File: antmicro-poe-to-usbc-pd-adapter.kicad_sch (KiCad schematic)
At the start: 93 parts, among them J1 Bus_RJ45_5-2337992-8, J2 Bus_RJ45_5-2337992-8, J3 USB-C_GCT_USB4105-GF-A, Q1 PJE138K, U1 TPS2372-3RGWR, U2 LV14540DDAR, U3 INA230AIRGTR, U4 IEA48003A280V-001-R, U5 FT4232H_VQFN, U6 TPS65987DDHRSHR, U7 LV14540DDAR, Y1 Resonator_12MHz_ABM8G

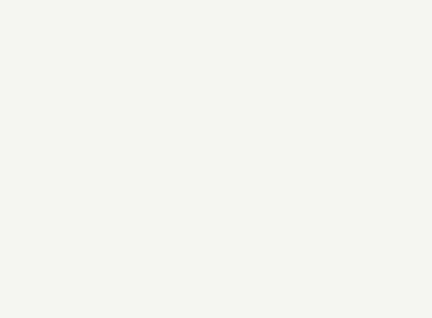
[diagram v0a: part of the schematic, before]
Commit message: [#62182] Change R5
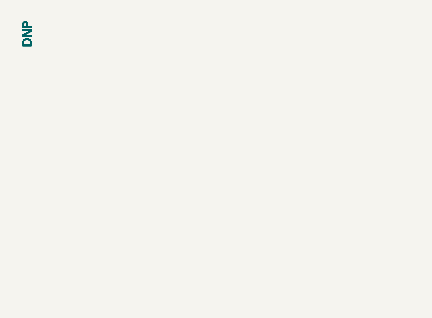
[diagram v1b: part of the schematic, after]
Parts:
- C2, R33, R34, R35, R36, R37, R38, R39, R40: DNP (none) -> DNP; now left out of the parts list
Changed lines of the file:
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@@
     (company "Antmicro ltd.")
   )
-  (bus_alias "CC" (members "CC1" "CC2"))
-  (bus_alias "ETH" (members "P1" "P2" "P3" "P6" "P7" "P8" "P9" "P10" "P4" "P5"))
-  (bus_alias "POE" (members "VC1" "VC2" "VC3" "VC4"))
   (junction (at 34.29 328.93) (diameter 0) (color 0 0 0 0)
   )
@@
     (stroke (width 0) (type default))
   )
+  (bus_alias "CC" (members "CC1" "CC2"))
+  (bus_alias "ETH" (members "P1" "P2" "P3" "P6" "P7" "P8" "P9" "P10" "P4" "P5"))
+  (bus_alias "POE" (members "VC1" "VC2" "VC3" "VC4"))
   (wire (pts (xy 317.5 292.735) (xy 321.945 292.735))
     (stroke (width 0) (type default))
@@
   )
   (symbol (lib_name "R_0R_0402_2") (lib_id "antmicroResistors0402:R_0R_0402") (at 317.5 292.735 90) (unit 1)
-    (in_bom yes) (on_board yes) (dnp yes)
+    (in_bom no) (on_board yes) (dnp yes)
     (property "Reference" "R40" (at 315.595 288.29 0)
       (effects (font (size 1.27 1.27) (thickness 0.15)) (justify right))
@@
       (effects (font (size 1.27 1.27) (thickness 0.15)) (justify left bottom) hide)
     )
+    (property "DNP" "DNP" (at 0.0 0.0 0)
+      (effects (font (size 1.0 1.0)))
+    )
     (pin "1")
     (pin "2")
@@
   )
   (symbol (lib_name "R_0R_0402_2") (lib_id "antmicroResistors0402:R_0R_0402") (at 292.735 299.72 90) (unit 1)
-    (in_bom yes) (on_board yes) (dnp yes)
+    (in_bom no) (on_board yes) (dnp yes)
     (property "Reference" "R36" (at 290.195 295.91 0)
       (effects (font (size 1.27 1.27) (thickness 0.15)) (justify right))
@@
       (effects (font (size 1.27 1.27) (thickness 0.15)) (justify left bottom) hide)
     )
+    (property "DNP" "DNP" (at 0.0 0.0 0)
+      (effects (font (size 1.0 1.0)))
+    )
     (pin "1")
     (pin "2")
@@
   )
   (symbol (lib_id "antmicroCapacitors0402:C_10n_50V_X7R_0402") (at 246.38 119.38 90) (unit 1)
-    (in_bom yes) (on_board yes) (dnp yes) (fields_autoplaced)
+    (in_bom no) (on_board yes) (dnp yes) (fields_autoplaced)
     (property "Reference" "C2" (at 248.92 115.5636 90)
       (effects (font (size 1.27 1.27) (thickness 0.15)) (justify right))
@@
       (effects (font (size 1.27 1.27) (thickness 0.15)) (justify left bottom) hide)
     )
+    (property "DNP" "DNP" (at 0.0 0.0 0)
+      (effects (font (size 1.0 1.0)))
+    )
     (pin "2")
     (pin "1")
@@
   )
   (symbol (lib_name "R_0R_0402_2") (lib_id "antmicroResistors0402:R_0R_0402") (at 297.18 293.37 90) (unit 1)
-    (in_bom yes) (on_board yes) (dnp yes)
+    (in_bom no) (on_board yes) (dnp yes)
     (property "Reference" "R35" (at 295.275 288.925 0)
       (effects (font (size 1.27 1.27) (thickness 0.15)) (justify right))
@@
       (effects (font (size 1.27 1.27) (thickness 0.15)) (justify left bottom) hide)
     )
+    (property "DNP" "DNP" (at 0.0 0.0 0)
+      (effects (font (size 1.0 1.0)))
+    )
     (pin "1")
     (pin "2")
@@
   )
   (symbol (lib_name "R_0R_0402_2") (lib_id "antmicroResistors0402:R_0R_0402") (at 313.69 299.085 90) (unit 1)
-    (in_bom yes) (on_board yes) (dnp yes)
+    (in_bom no) (on_board yes) (dnp yes)
     (property "Reference" "R39" (at 311.15 295.275 0)
       (effects (font (size 1.27 1.27) (thickness 0.15)) (justify right))
@@
       (effects (font (size 1.27 1.27) (thickness 0.15)) (justify left bottom) hide)
     )
+    (property "DNP" "DNP" (at 0.0 0.0 0)
+      (effects (font (size 1.0 1.0)))
+    )
     (pin "1")
     (pin "2")
@@
   )
   (symbol (lib_name "R_0R_0402_2") (lib_id "antmicroResistors0402:R_0R_0402") (at 288.925 293.37 90) (unit 1)
-    (in_bom yes) (on_board yes) (dnp yes)
+    (in_bom no) (on_board yes) (dnp yes)
     (property "Reference" "R33" (at 287.02 288.925 0)
       (effects (font (size 1.27 1.27) (thickness 0.15)) (justify right))
@@
       (effects (font (size 1.27 1.27) (thickness 0.15)) (justify left bottom) hide)
     )
+    (property "DNP" "DNP" (at 0.0 0.0 0)
+      (effects (font (size 1.0 1.0)))
+    )
     (pin "1")
     (pin "2")
@@
   )
   (symbol (lib_name "R_0R_0402_2") (lib_id "antmicroResistors0402:R_0R_0402") (at 313.69 292.735 90) (unit 1)
-    (in_bom yes) (on_board yes) (dnp yes)
+    (in_bom no) (on_board yes) (dnp yes)
     (property "Reference" "R38" (at 311.785 288.29 0)
       (effects (font (size 1.27 1.27) (thickness 0.15)) (justify right))
@@
       (effects (font (size 1.27 1.27) (thickness 0.15)) (justify left bottom) hide)
     )
+    (property "DNP" "DNP" (at 0.0 0.0 0)
+      (effects (font (size 1.0 1.0)))
+    )
     (pin "1")
     (pin "2")
@@
   )
   (symbol (lib_name "R_0R_0402_2") (lib_id "antmicroResistors0402:R_0R_0402") (at 309.88 292.735 90) (unit 1)
-    (in_bom yes) (on_board yes) (dnp yes)
+    (in_bom no) (on_board yes) (dnp yes)
     (property "Reference" "R37" (at 307.975 288.29 0)
       (effects (font (size 1.27 1.27) (thickness 0.15)) (justify right))
@@
       (effects (font (size 1.27 1.27) (thickness 0.15)) (justify left bottom) hide)
     )
+    (property "DNP" "DNP" (at 0.0 0.0 0)
+      (effects (font (size 1.0 1.0)))
+    )
     (pin "1")
     (pin "2")
@@
   )
   (symbol (lib_name "R_0R_0402_2") (lib_id "antmicroResistors0402:R_0R_0402") (at 292.735 293.37 90) (unit 1)
-    (in_bom yes) (on_board yes) (dnp yes)
+    (in_bom no) (on_board yes) (dnp yes)
     (property "Reference" "R34" (at 290.83 288.925 0)
       (effects (font (size 1.27 1.27) (thickness 0.15)) (justify right))
@@
       (effects (font (size 1.27 1.27) (thickness 0.15)) (justify left bottom) hide)
     )
+    (property "DNP" "DNP" (at 0.0 0.0 0)
+      (effects (font (size 1.0 1.0)))
+    )
     (pin "1")
